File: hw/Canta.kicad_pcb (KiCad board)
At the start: 2 copper layers, 85.6 x 54 mm, 49 parts, among them J1 USB_C_Receptacle_PowerOnly_6P, J101 Conn_01x01, J102 Conn_01x01, J103 Conn_01x01, J104 Conn_01x01, J105 Conn_01x01, J106 Conn_01x01, J107 Conn_01x01, J108 Conn_01x01, J109 Conn_01x01, J110 Conn_01x01, J111 Conn_01x01, J112 Conn_01x01, J2 Conn_01x03, U2 PY32F003F18U6, U3 TM8211, U4 FM8002A, Y1 32MHz 12pF

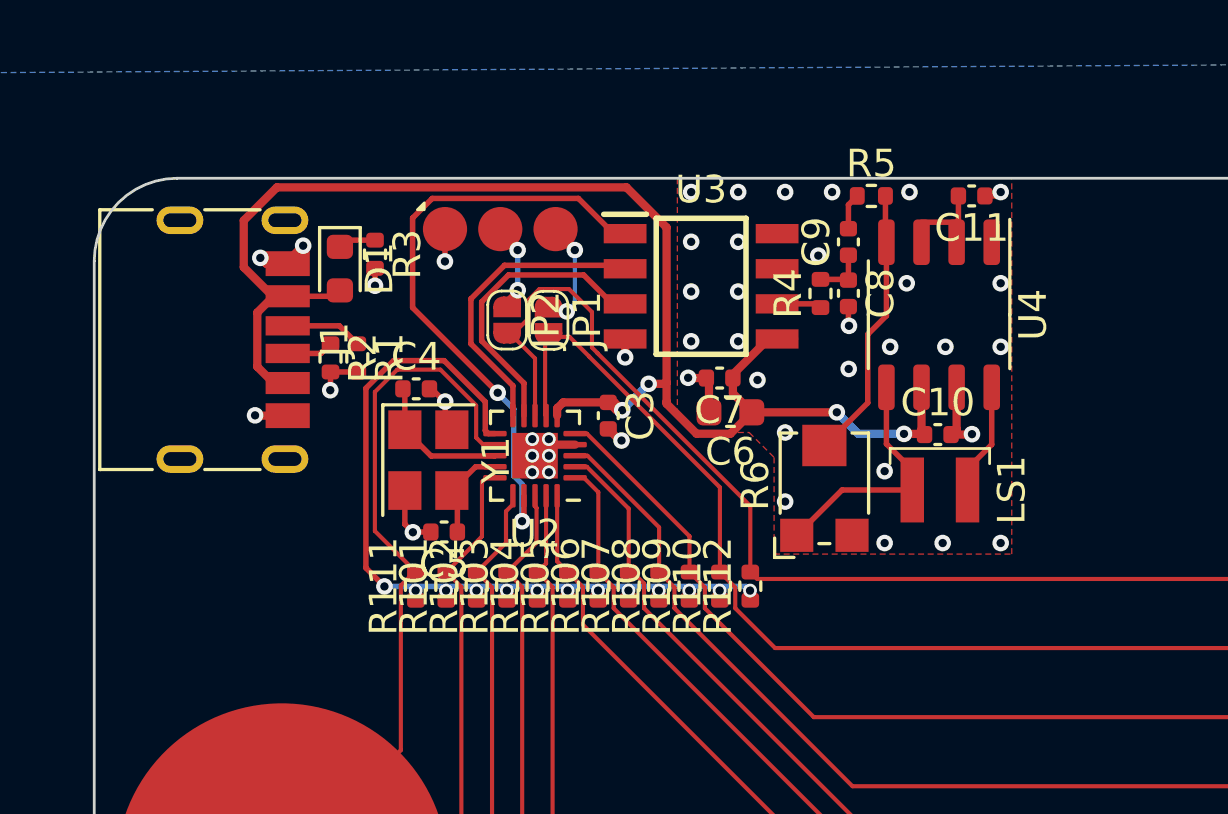
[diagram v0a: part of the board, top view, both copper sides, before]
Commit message: Update silkscreen
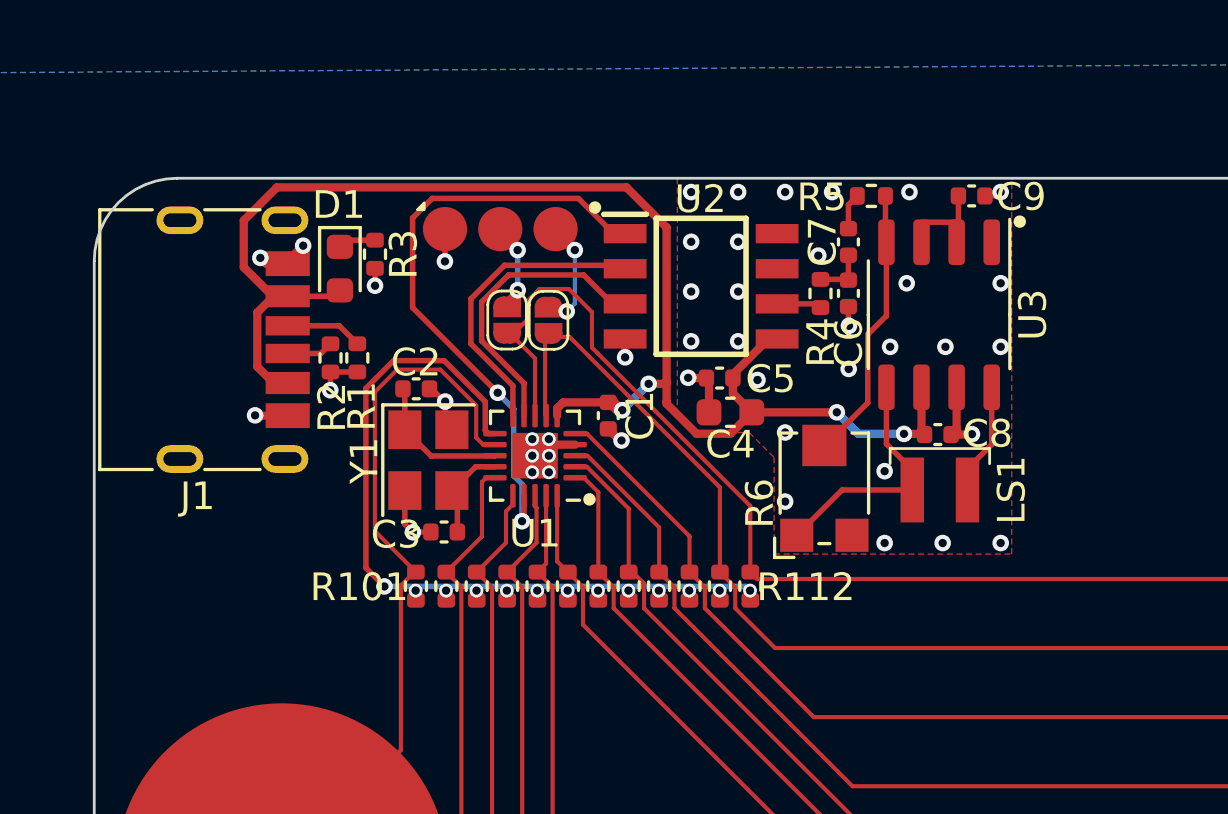
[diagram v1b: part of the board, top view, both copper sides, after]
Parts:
- R3: value 7.5k -> 10k
- renumbered C3 to C1, C4 to C2, C5 to C3, C6 to C4, C7 to C5, C8 to C6, C9 to C7, C10 to C8, C11 to C9, U2 to U1, U3 to U2, U4 to U3
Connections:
- C2 pad 1: Net-(U2-PF0) -> (no net)
- C3 pad 1: Net-(U2-PF1) -> (no net)
- C6 pad 1: Net-(C8-Pad1) -> (no net)
- C7 pad 1: Net-(C8-Pad1) -> Net-(C6-Pad1)
- C7 pad 2: Net-(C9-Pad2) -> (no net)
- C9 pad 2: Net-(U4-+IN) -> (no net)
- R4 pad 2: Net-(C8-Pad1) -> Net-(C6-Pad1)
- R5 pad 1: Net-(C9-Pad2) -> Net-(C7-Pad2)
- U1 pad 13: Net-(U2-PF0) -> Net-(U1-PF0)
- U1 pad 14: Net-(U2-PF1) -> Net-(U1-PF1)
- U2 pad 7: unconnected-(U3-NC-Pad7) -> (no net)
- U2 pad 8: unconnected-(U3-RCH-Pad8) -> (no net)
- U3 pad 1: unconnected-(U4-SD-Pad1) -> (no net)
- U3 pad 2: Net-(U4-+IN) -> Net-(U3-+IN)
- U3 pad 3: Net-(U4-+IN) -> Net-(U3-+IN)
- Y1 pad 1: Net-(U2-PF0) -> Net-(U1-PF0)
- Y1 pad 3: Net-(U2-PF1) -> Net-(U1-PF1)
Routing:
- net Net-(U2-PF0): track 5.17 -> 0.00 mm
- net Net-(U1-PF0): track 0.00 -> 5.17 mm
- net Net-(U2-PF1): track 3.50 -> 0.00 mm
- net Net-(U1-PF1): track 0.00 -> 3.50 mm
- net Net-(U4-+IN): track 2.97 -> 0.00 mm
- net Net-(U3-+IN): track 0.00 -> 2.97 mm
- net Net-(C8-Pad1): track 1.92 -> 0.00 mm
- net Net-(C6-Pad1): track 0.00 -> 1.92 mm
- net Net-(C9-Pad2): track 1.32 -> 0.00 mm
- net Net-(C7-Pad2): track 0.00 -> 1.32 mm
